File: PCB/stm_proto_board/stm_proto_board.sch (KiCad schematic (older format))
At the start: 41 parts, among them J1 Conn_01x08, J10 Conn_01x02, J11 Conn_01x04, J12 Conn_01x04, J13 Conn_01x04, J14 Conn_01x08, J15 Conn_01x02, J2 Conn_01x04, J3 DB9_Female, J4 Conn_01x02, J5 Conn_01x04, J6 Conn_01x02, J7 Conn_01x04, J8 Conn_01x04, J9 Conn_01x04, SW1 SW_Push, SW2 SW_Push, SW3 SW_Push, SW4 SW_Push, U1 YAAJ_BluePill_Part_Like, U2 MCP2551-I-P, U3 MAX3232_convertor, U4 LTV-814, U5 L7805, U6 4N25, U7 4N25, U8 4N25, U9 4N25

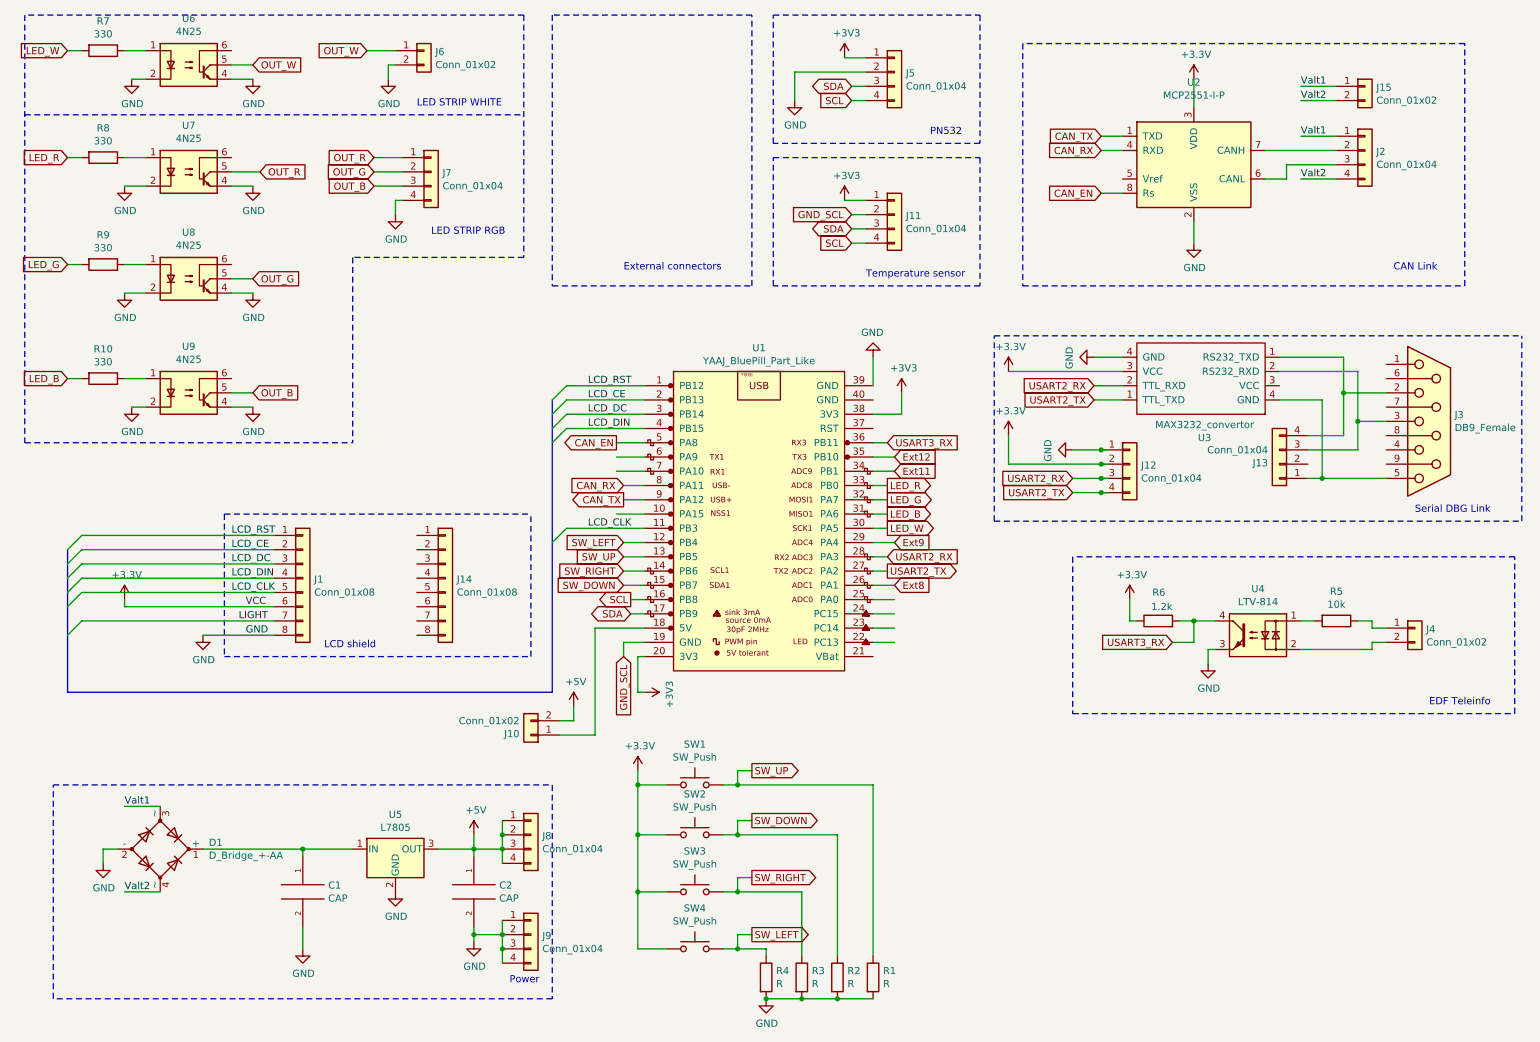
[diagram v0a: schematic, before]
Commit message: update PCB
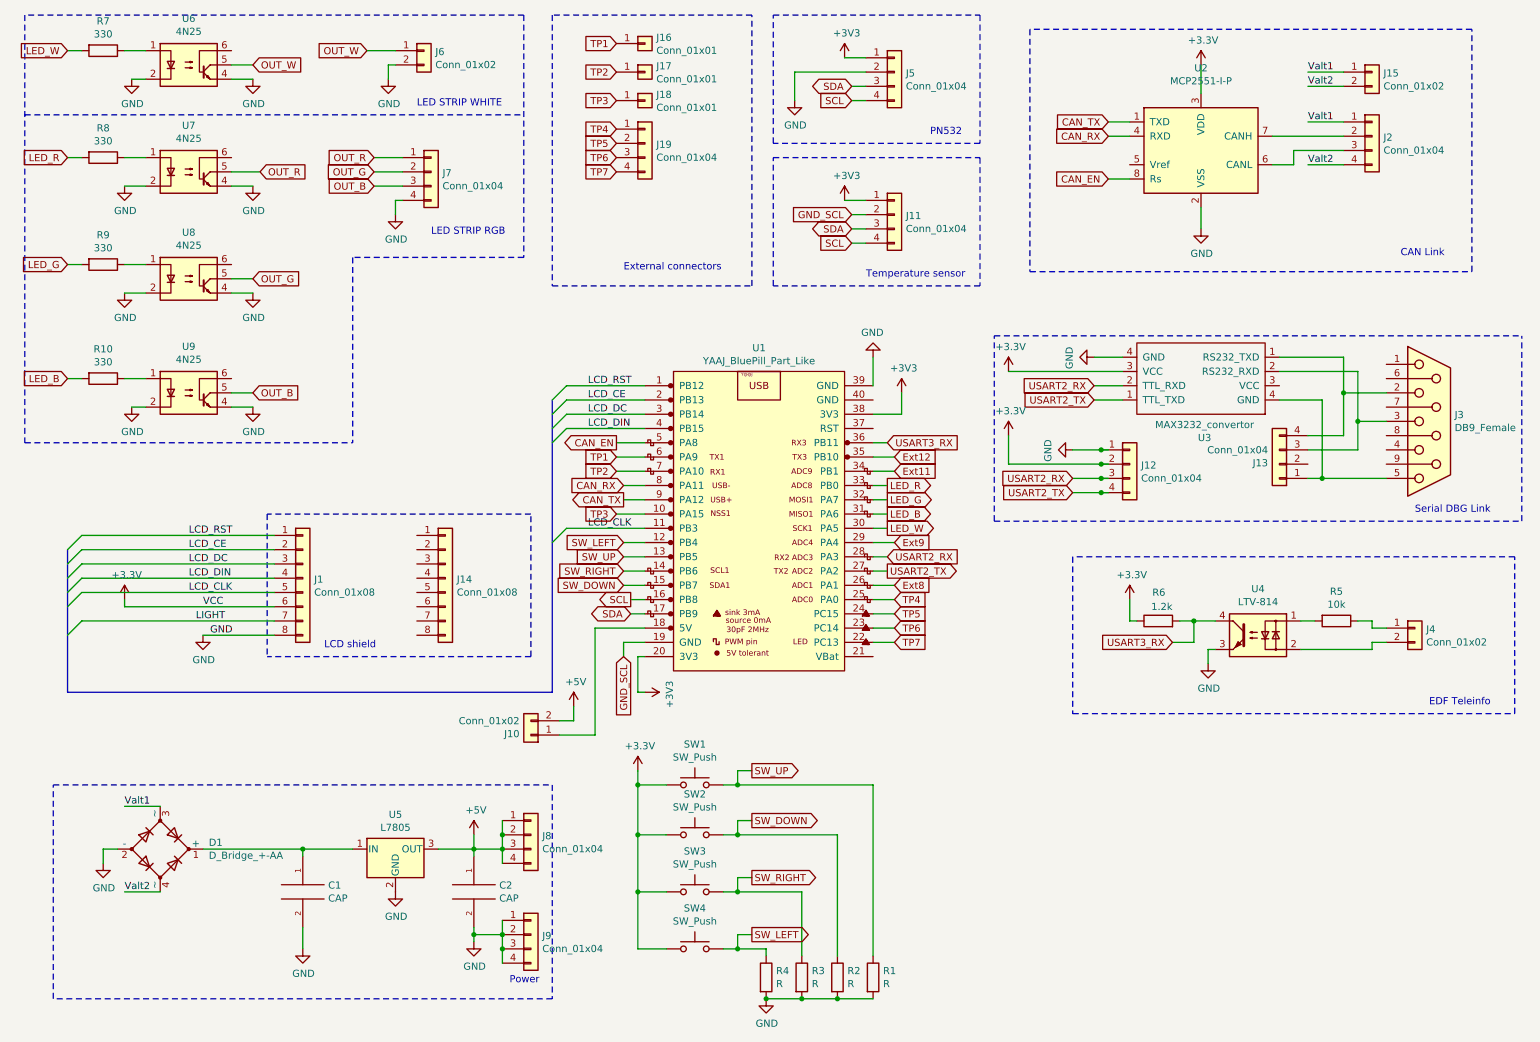
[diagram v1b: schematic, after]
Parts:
- added J16, J17, J18: Conn_01x01, Connector_PinHeader_2.54mm:PinHeader_1x01_P2.54mm_Vertical, symbol Connector_Generic:Conn_01x01
- added J19: Conn_01x04, Connector_PinHeader_2.54mm:PinHeader_1x04_P2.54mm_Vertical, symbol Connector_Generic:Conn_01x04
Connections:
- net labels added: TP1, TP2, TP3, TP4, TP5, TP6, TP7
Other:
- moved on the sheet: J15, J2, U2
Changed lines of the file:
@@
 L Interface_CAN_LIN:MCP2551-I-P U2
 U 1 1 5B6EF31C
-P 8800 1650
-F 0 "U2" H 8800 2228 50  0000 C CNN
-F 1 "MCP2551-I-P" H 8800 2137 50  0000 C CNN
-F 2 "Package_DIP:DIP-8_W7.62mm" H 8800 1150 50  0001 C CIN
-F 3 "http://ww1.microchip.com/downloads/en/devicedoc/21667d.pdf" H 8800 1650 50  0001 C CNN
-	1    8800 1650
+P 8850 1550
+F 0 "U2" H 8850 2128 50  0000 C CNN
+F 1 "MCP2551-I-P" H 8850 2037 50  0000 C CNN
+F 2 "Package_DIP:DIP-8_W7.62mm" H 8850 1050 50  0001 C CIN
+F 3 "http://ww1.microchip.com/downloads/en/devicedoc/21667d.pdf" H 8850 1550 50  0001 C CNN
+	1    8850 1550
 	1    0    0    -1
 $EndComp
@@
 L Connector_Generic:Conn_01x04 J2
 U 1 1 5B6EF715
-P 10000 1550
-F 0 "J2" H 10080 1542 50  0000 L CNN
-F 1 "Conn_01x04" H 10080 1451 50  0000 L CNN
-F 2 "Connector_PinHeader_2.54mm:PinHeader_1x04_P2.54mm_Horizontal" H 10000 1550 50  0001 C CNN
-F 3 "~" H 10000 1550 50  0001 C CNN
-	1    10000 1550
+P 10050 1450
+F 0 "J2" H 10130 1442 50  0000 L CNN
+F 1 "Conn_01x04" H 10130 1351 50  0000 L CNN
+F 2 "Connector_PinHeader_2.54mm:PinHeader_1x04_P2.54mm_Horizontal" H 10050 1450 50  0001 C CNN
+F 3 "~" H 10050 1450 50  0001 C CNN
+	1    10050 1450
 	1    0    0    -1
 $EndComp
@@
 L power:+3.3V #PWR0105
 U 1 1 5B6EE504
-P 8800 1050
-F 0 "#PWR0105" H 8800 900 50  0001 C CNN
-F 1 "+3.3V" H 8815 1223 50  0000 C CNN
-F 2 "" H 8800 1050 50  0001 C CNN
-F 3 "" H 8800 1050 50  0001 C CNN
-	1    8800 1050
-	1    0    0    -1
-$EndComp
-Wire Wire Line
-	8800 1250 8800 1050
+P 8850 950
+F 0 "#PWR0105" H 8850 800 50  0001 C CNN
+F 1 "+3.3V" H 8865 1123 50  0000 C CNN
+F 2 "" H 8850 950 50  0001 C CNN
+F 3 "" H 8850 950 50  0001 C CNN
+	1    8850 950
+	1    0    0    -1
+$EndComp
+Wire Wire Line
+	8850 1150 8850 950
 $Comp
 L power:GND #PWR0106
 U 1 1 5B6EE5EC
-P 8800 2200
-F 0 "#PWR0106" H 8800 1950 50  0001 C CNN
-F 1 "GND" H 8805 2027 50  0000 C CNN
-F 2 "" H 8800 2200 50  0001 C CNN
-F 3 "" H 8800 2200 50  0001 C CNN
-	1    8800 2200
-	1    0    0    -1
-$EndComp
-Wire Wire Line
-	8800 2050 8800 2200
-Wire Wire Line
-	9800 1550 9300 1550
-Wire Wire Line
-	9300 1750 9450 1750
-Wire Wire Line
-	9450 1750 9450 1650
-Wire Wire Line
-	9450 1650 9800 1650
-Text Label 9550 1450 0    50   ~ 0
+P 8850 2100
+F 0 "#PWR0106" H 8850 1850 50  0001 C CNN
+F 1 "GND" H 8855 1927 50  0000 C CNN
+F 2 "" H 8850 2100 50  0001 C CNN
+F 3 "" H 8850 2100 50  0001 C CNN
+	1    8850 2100
+	1    0    0    -1
+$EndComp
+Wire Wire Line
+	8850 1950 8850 2100
+Wire Wire Line
+	9850 1450 9350 1450
+Wire Wire Line
+	9350 1650 9500 1650
+Wire Wire Line
+	9500 1650 9500 1550
+Wire Wire Line
+	9500 1550 9850 1550
+Text Label 9600 1350 0    50   ~ 0
 Valt1
 Wire Wire Line
-	9550 1450 9800 1450
-Text Label 9550 1750 0    50   ~ 0
+	9600 1350 9850 1350
+Text Label 9600 1650 0    50   ~ 0
 Valt2
 Wire Wire Line
-	9550 1750 9800 1750
-Text Label 2050 4250 0    50   ~ 0
+	9600 1650 9850 1650
+Text Label 1750 4250 0    50   ~ 0
 LCD_RST
-Text Label 2050 4350 0    50   ~ 0
+Text Label 1750 4350 0    50   ~ 0
 LCD_CE
-Text Label 2050 4450 0    50   ~ 0
+Text Label 1750 4450 0    50   ~ 0
 LCD_DC
-Text Label 2050 4550 0    50   ~ 0
+Text Label 1750 4550 0    50   ~ 0
 LCD_DIN
-Text Label 2050 4650 0    50   ~ 0
+Text Label 1750 4650 0    50   ~ 0
 LCD_CLK
-Text Label 2150 4750 0    50   ~ 0
+Text Label 1850 4750 0    50   ~ 0
 VCC
-Text Label 2100 4850 0    50   ~ 0
+Text Label 1800 4850 0    50   ~ 0
 LIGHT
-Text Label 2150 4950 0    50   ~ 0
+Text Label 1900 4950 0    50   ~ 0
 GND
 $Comp
@@
 Wire Wire Line
 	1300 4750 2350 4750
-Text GLabel 8150 1450 0    50   Input ~ 0
+Text GLabel 8200 1350 0    50   Input ~ 0
 CAN_TX
-Text GLabel 8150 1550 0    50   Input ~ 0
+Text GLabel 8200 1450 0    50   Input ~ 0
 CAN_RX
-Text GLabel 8150 1850 0    50   Input ~ 0
+Text GLabel 8200 1750 0    50   Input ~ 0
 CAN_EN
 Wire Wire Line
-	8300 1450 8150 1450
-Wire Wire Line
-	8300 1550 8150 1550
-Wire Wire Line
-	8150 1850 8300 1850
+	8350 1350 8200 1350
+Wire Wire Line
+	8350 1450 8200 1450
+Wire Wire Line
+	8200 1750 8350 1750
 Entry Wire Line
 	1000 4450 900  4550
@@
 EDF Teleinfo
 Wire Notes Line
-	7600 2500 10700 2500
-Wire Notes Line
-	10700 2500 10700 800
-Wire Notes Line
-	10700 800  7600 800
-Wire Notes Line
-	7600 800  7600 2500
-Text Notes 10200 2400 0    50   ~ 0
+	7650 2400 10750 2400
+Wire Notes Line
+	10750 2400 10750 700
+Wire Notes Line
+	10750 700  7650 700
+Wire Notes Line
+	7650 700  7650 2400
+Text Notes 10250 2300 0    50   ~ 0
 CAN Link
 Wire Notes Line
-	2000 4100 2000 5100
+	2300 4100 2300 5100
 Wire Notes Line
 	4150 5100 4150 4100
@@
 Wire Wire Line
 	6550 4200 6650 4200
-Text Label 9550 1100 0    50   ~ 0
+Text Label 9600 1000 0    50   ~ 0
 Valt1
 Wire Wire Line
-	9550 1100 9800 1100
-Text Label 9550 1200 0    50   ~ 0
+	9600 1000 9850 1000
+Text Label 9600 1100 0    50   ~ 0
 Valt2
 Wire Wire Line
-	9550 1200 9800 1200
+	9600 1100 9850 1100
 $Comp
 L Connector_Generic:Conn_01x02 J15
 U 1 1 603342BF
-P 10000 1100
-F 0 "J15" H 10080 1092 50  0000 L CNN
-F 1 "Conn_01x02" H 10080 1001 50  0000 L CNN
-F 2 "Connector_PinHeader_2.54mm:PinHeader_1x02_P2.54mm_Vertical" H 10000 1100 50  0001 C CNN
-F 3 "~" H 10000 1100 50  0001 C CNN
-	1    10000 1100
+P 10050 1000
+F 0 "J15" H 10130 992 50  0000 L CNN
+F 1 "Conn_01x02" H 10130 901 50  0000 L CNN
+F 2 "Connector_PinHeader_2.54mm:PinHeader_1x02_P2.54mm_Vertical" H 10050 1000 50  0001 C CNN
+F 3 "~" H 10050 1000 50  0001 C CNN
+	1    10050 1000
 	1    0    0    -1
 $EndComp
@@
 	1    0    0    -1
 $EndComp
-Wire Notes Line
-	2000 4100 4150 4100
-Wire Notes Line
-	2000 5100 4150 5100
 Wire Wire Line
 	4950 4400 4800 4400
@@
 Wire Wire Line
 	4800 5000 4800 5100
+$Comp
+L Connector_Generic:Conn_01x01 J16
+U 1 1 5F91D967
+P 4950 800
+F 0 "J16" H 5030 842 50  0000 L CNN
+F 1 "Conn_01x01" H 5030 751 50  0000 L CNN
+F 2 "Connector_PinHeader_2.54mm:PinHeader_1x01_P2.54mm_Vertical" H 4950 800 50  0001 C CNN
+F 3 "~" H 4950 800 50  0001 C CNN
+	1    4950 800
+	1    0    0    -1
+$EndComp
+$Comp
+L Connector_Generic:Conn_01x01 J17
+U 1 1 5F924708
+P 4950 1000
+F 0 "J17" H 5030 1042 50  0000 L CNN
+F 1 "Conn_01x01" H 5030 951 50  0000 L CNN
+F 2 "Connector_PinHeader_2.54mm:PinHeader_1x01_P2.54mm_Vertical" H 4950 1000 50  0001 C CNN
+F 3 "~" H 4950 1000 50  0001 C CNN
+	1    4950 1000
+	1    0    0    -1
+$EndComp
+$Comp
+L Connector_Generic:Conn_01x01 J18
+U 1 1 5F932C0D
+P 4950 1200
+F 0 "J18" H 5030 1242 50  0000 L CNN
+F 1 "Conn_01x01" H 5030 1151 50  0000 L CNN
+F 2 "Connector_PinHeader_2.54mm:PinHeader_1x01_P2.54mm_Vertical" H 4950 1200 50  0001 C CNN
+F 3 "~" H 4950 1200 50  0001 C CNN
+	1    4950 1200
+	1    0    0    -1
+$EndComp
+Text GLabel 4750 800  0    50   Input ~ 0
+TP1
+Text GLabel 4750 1000 0    50   Input ~ 0
+TP2
+Text GLabel 4750 1200 0    50   Input ~ 0
+TP3
+Text GLabel 4750 1400 0    50   Input ~ 0
+TP4
+Text GLabel 4750 3700 0    50   Input ~ 0
+TP1
+Text GLabel 4750 3800 0    50   Input ~ 0
+TP2
+Text GLabel 4750 4100 0    50   Input ~ 0
+TP3
+Text GLabel 4750 1500 0    50   Input ~ 0
+TP5
+Text GLabel 4750 1600 0    50   Input ~ 0
+TP6
+Text GLabel 6700 4700 2    50   Input ~ 0
+TP4
+Text GLabel 6700 4800 2    50   Input ~ 0
+TP5
+Text GLabel 6700 4900 2    50   Input ~ 0
+TP6
+Text GLabel 4750 1700 0    50   Input ~ 0
+TP7
+Text GLabel 6700 5000 2    50   Input ~ 0
+TP7
+$Comp
+L Connector_Generic:Conn_01x04 J19
+U 1 1 5FBFD4E3
+P 4950 1500
+F 0 "J19" H 5030 1492 50  0000 L CNN
+F 1 "Conn_01x04" H 5030 1401 50  0000 L CNN
+F 2 "Connector_PinHeader_2.54mm:PinHeader_1x04_P2.54mm_Vertical" H 4950 1500 50  0001 C CNN
+F 3 "~" H 4950 1500 50  0001 C CNN
+	1    4950 1500
+	1    0    0    -1
+$EndComp
+Wire Notes Line
+	4150 4100 2300 4100
+Wire Notes Line
+	4150 5100 2300 5100
 Wire Bus Line
 	4300 3300 4300 5350
